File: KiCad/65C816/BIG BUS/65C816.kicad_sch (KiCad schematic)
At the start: 34 parts, among them J1 Expansion Bus, J2 Expansion Bus, J3 Expansion Bus, J4 Expansion Bus, J5 Expansion Bus, J6 Expansion Bus, J7 Displays, J8 Serial, J9 PWR IN, SW2 RESET, SW3 PWR_ON, U1 W65C816SxP, U10 74LS109, U2 HM62256BLP, U3 74HC00, U4 28C256, U5 ATF16V8B, U6 74HC245, U7 74LS573, U8 NE555P, U9 74LS109, Y1 16MHz

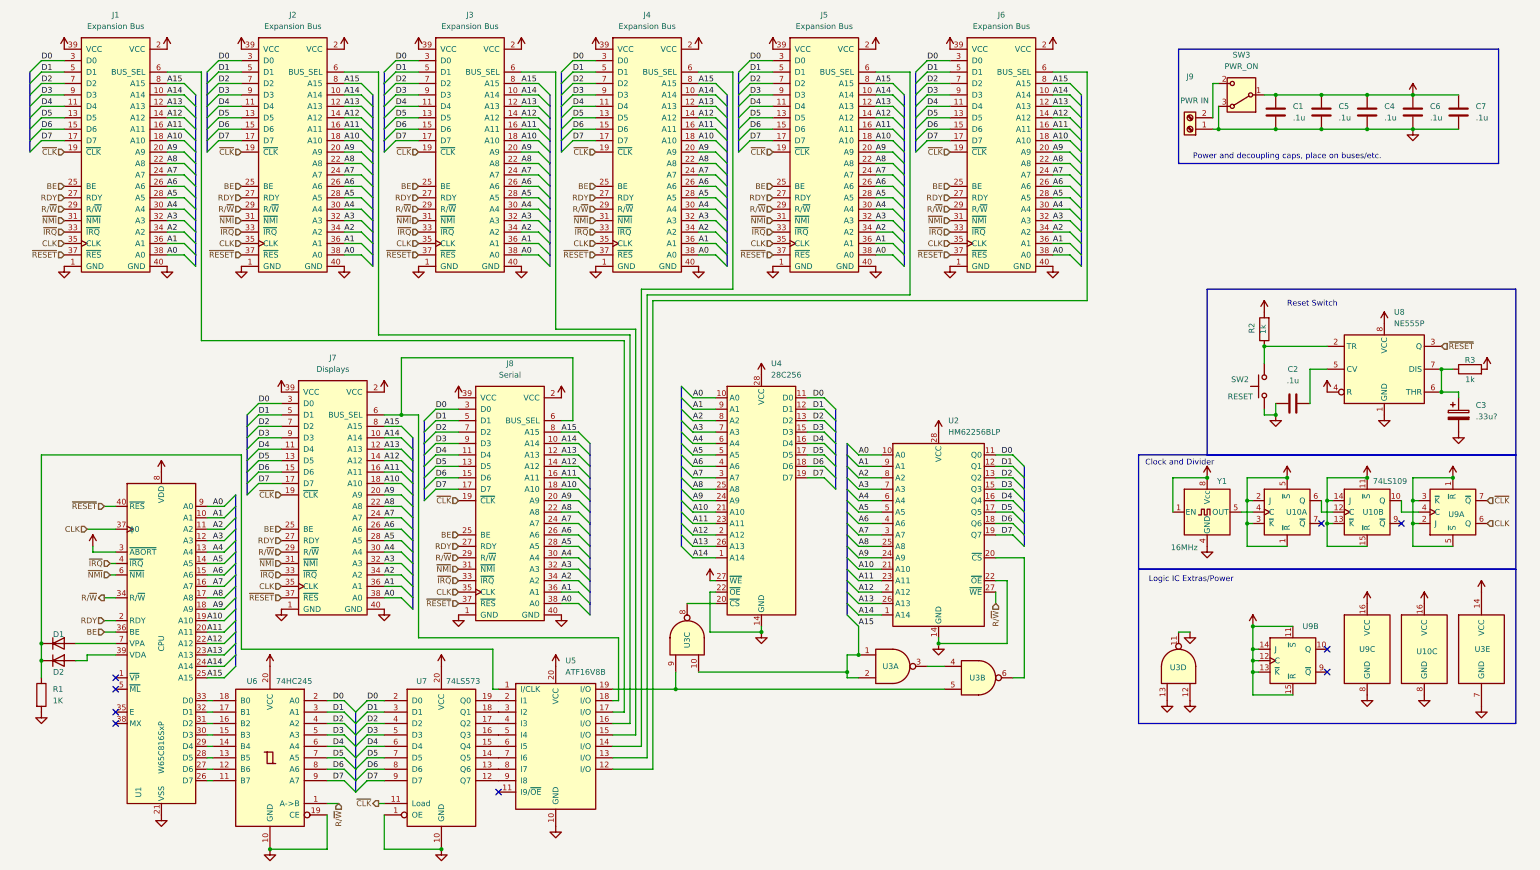
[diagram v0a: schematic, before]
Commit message: Cleaned up random files, added actual .gitignore on my end lmao
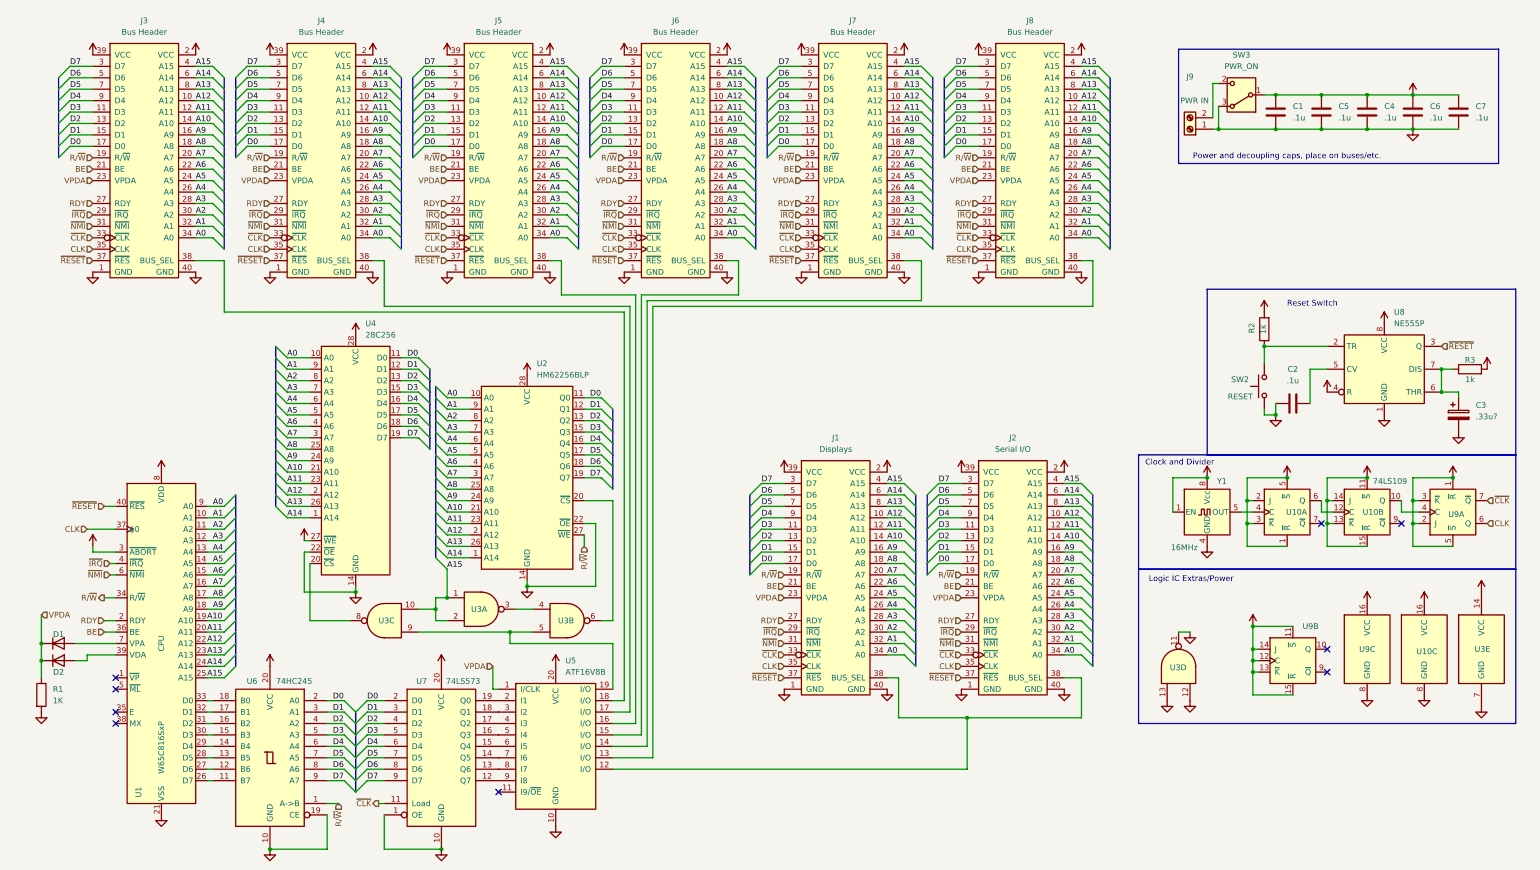
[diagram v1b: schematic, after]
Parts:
- removed J1, J2, J3, J4, J5, J6: Expansion Bus, Connector_IDC:IDC-Header_2x20_P2.54mm_Vertical, symbol Board Connectors:Generic Board Connector
- removed J7: Displays, Connector_IDC:IDC-Header_2x20_P2.54mm_Vertical, symbol Board Connectors:Generic Board Connector
- removed J8: Serial, Connector_IDC:IDC-Header_2x20_P2.54mm_Vertical, symbol Board Connectors:Generic Board Connector
- added J1: Displays, Connector_IDC:IDC-Header_2x20_P2.54mm_Vertical, symbol Board Connectors:Board_Bus_V2
- added J2: Serial I/O, Connector_IDC:IDC-Header_2x20_P2.54mm_Vertical, symbol Board Connectors:Board_Bus_V2
- added J3, J4, J5, J6, J7, J8: Bus Header, Connector_IDC:IDC-Header_2x20_P2.54mm_Vertical, symbol Board Connectors:Board_Bus_V2
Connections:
- net +5V: now also J1.2 (VCC), J1.39 (VCC), J2.2 (VCC), J2.39 (VCC), J3.2 (VCC), J3.39 (VCC), J4.2 (VCC), J4.39 (VCC), J5.2 (VCC), J5.39 (VCC), J6.2 (VCC), J6.39 (VCC), J7.2 (VCC), J7.39 (VCC), J8.2 (VCC), J8.39 (VCC)
- net A0: now also J1.34 (A0), J2.34 (A0), J3.34 (A0), J4.34 (A0), J5.34 (A0), J6.34 (A0), J7.34 (A0), J8.34 (A0)
- net A1: now also J1.32 (A1), J2.32 (A1), J3.32 (A1), J4.32 (A1), J5.32 (A1), J6.32 (A1), J7.32 (A1), J8.32 (A1)
- net A10: now also J1.14 (A10), J2.14 (A10), J3.14 (A10), J4.14 (A10), J5.14 (A10), J6.14 (A10), J7.14 (A10), J8.14 (A10)
- net A11: now also J1.12 (A11), J2.12 (A11), J3.12 (A11), J4.12 (A11), J5.12 (A11), J6.12 (A11), J7.12 (A11), J8.12 (A11)
- net A12: now also J1.10 (A12), J2.10 (A12), J3.10 (A12), J4.10 (A12), J5.10 (A12), J6.10 (A12), J7.10 (A12), J8.10 (A12)
- net A13: now also J1.8 (A13), J2.8 (A13), J3.8 (A13), J4.8 (A13), J5.8 (A13), J6.8 (A13), J7.8 (A13), J8.8 (A13)
- net A14: now also J1.6 (A14), J2.6 (A14), J3.6 (A14), J4.6 (A14), J5.6 (A14), J6.6 (A14), J7.6 (A14), J8.6 (A14)
- net A15: now also J1.4 (A15), J2.4 (A15), J3.4 (A15), J4.4 (A15), J5.4 (A15), J6.4 (A15), J7.4 (A15), J8.4 (A15)
- net A2: now also J1.30 (A2), J2.30 (A2), J3.30 (A2), J4.30 (A2), J5.30 (A2), J6.30 (A2), J7.30 (A2), J8.30 (A2)
- net A3: now also J1.28 (A3), J2.28 (A3), J3.28 (A3), J4.28 (A3), J5.28 (A3), J6.28 (A3), J7.28 (A3), J8.28 (A3)
- net A4: now also J1.26 (A4), J2.26 (A4), J3.26 (A4), J4.26 (A4), J5.26 (A4), J6.26 (A4), J7.26 (A4), J8.26 (A4)
- net A5: now also J1.24 (A5), J2.24 (A5), J3.24 (A5), J4.24 (A5), J5.24 (A5), J6.24 (A5), J7.24 (A5), J8.24 (A5)
- net A6: now also J1.22 (A6), J2.22 (A6), J3.22 (A6), J4.22 (A6), J5.22 (A6), J6.22 (A6), J7.22 (A6), J8.22 (A6)
- net A7: now also J1.20 (A7), J2.20 (A7), J3.20 (A7), J4.20 (A7), J5.20 (A7), J6.20 (A7), J7.20 (A7), J8.20 (A7)
- net A8: now also J1.18 (A8), J2.18 (A8), J3.18 (A8), J4.18 (A8), J5.18 (A8), J6.18 (A8), J7.18 (A8), J8.18 (A8)
- net A9: now also J1.16 (A9), J2.16 (A9), J3.16 (A9), J4.16 (A9), J5.16 (A9), J6.16 (A9), J7.16 (A9), J8.16 (A9)
- net BE: now also J1.21 (BE), J2.21 (BE), J3.21 (BE), J4.21 (BE), J5.21 (BE), J6.21 (BE), J7.21 (BE), J8.21 (BE)
- net CLK: now also J1.35 (CLK), J2.35 (CLK), J3.35 (CLK), J4.35 (CLK), J5.35 (CLK), J6.35 (CLK), J7.35 (CLK), J8.35 (CLK)
- net D0: now also J1.17 (D0), J2.17 (D0), J3.17 (D0), J4.17 (D0), J5.17 (D0), J6.17 (D0), J7.17 (D0), J8.17 (D0)
- net D1: now also J1.15 (D1), J2.15 (D1), J3.15 (D1), J4.15 (D1), J5.15 (D1), J6.15 (D1), J7.15 (D1), J8.15 (D1)
- net D2: now also J1.13 (D2), J2.13 (D2), J3.13 (D2), J4.13 (D2), J5.13 (D2), J6.13 (D2), J7.13 (D2), J8.13 (D2)
- net D3: now also J1.11 (D3), J2.11 (D3), J3.11 (D3), J4.11 (D3), J5.11 (D3), J6.11 (D3), J7.11 (D3), J8.11 (D3)
- net D4: now also J1.9 (D4), J2.9 (D4), J3.9 (D4), J4.9 (D4), J5.9 (D4), J6.9 (D4), J7.9 (D4), J8.9 (D4)
- net D5: now also J1.7 (D5), J2.7 (D5), J3.7 (D5), J4.7 (D5), J5.7 (D5), J6.7 (D5), J7.7 (D5), J8.7 (D5)
- net D6: now also J1.5 (D6), J2.5 (D6), J3.5 (D6), J4.5 (D6), J5.5 (D6), J6.5 (D6), J7.5 (D6), J8.5 (D6)
- net D7: now also J1.3 (D7), J2.3 (D7), J3.3 (D7), J4.3 (D7), J5.3 (D7), J6.3 (D7), J7.3 (D7), J8.3 (D7)
- net GND: now also J1.1 (GND), J1.40 (GND), J2.1 (GND), J2.40 (GND), J3.1 (GND), J3.40 (GND), J4.1 (GND), J4.40 (GND), J5.1 (GND), J5.40 (GND), J6.1 (GND), J6.40 (GND), J7.1 (GND), J7.40 (GND), J8.1 (GND), J8.40 (GND)
- net RDY: now also J1.27 (RDY), J2.27 (RDY), J3.27 (RDY), J4.27 (RDY), J5.27 (RDY), J6.27 (RDY), J7.27 (RDY), J8.27 (RDY)
- net R/~{W}: now also J1.19 (R/~{W}), J2.19 (R/~{W}), J3.19 (R/~{W}), J4.19 (R/~{W}), J5.19 (R/~{W}), J6.19 (R/~{W}), J7.19 (R/~{W}), J8.19 (R/~{W})
- net ~{CLK}: now also J1.33 (~{CLK}), J2.33 (~{CLK}), J3.33 (~{CLK}), J4.33 (~{CLK}), J5.33 (~{CLK}), J6.33 (~{CLK}), J7.33 (~{CLK}), J8.33 (~{CLK})
- net ~{IRQ}: now also J1.29 (~{IRQ}), J2.29 (~{IRQ}), J3.29 (~{IRQ}), J4.29 (~{IRQ}), J5.29 (~{IRQ}), J6.29 (~{IRQ}), J7.29 (~{IRQ}), J8.29 (~{IRQ})
- net ~{NMI}: now also J1.31 (~{NMI}), J2.31 (~{NMI}), J3.31 (~{NMI}), J4.31 (~{NMI}), J5.31 (~{NMI}), J6.31 (~{NMI}), J7.31 (~{NMI}), J8.31 (~{NMI})
- net ~{RESET}: now also J1.37 (~{RES}), J2.37 (~{RES}), J3.37 (~{RES}), J4.37 (~{RES}), J5.37 (~{RES}), J6.37 (~{RES}), J7.37 (~{RES}), J8.37 (~{RES})
- net at U5.15 (I/O): now also J6.38 (BUS_SEL)
- net at U5.18 (I/O): now also J3.38 (BUS_SEL)
- net at U5.14 (I/O): now also J7.38 (BUS_SEL)
- net at U5.12 (I/O): now also J1.38 (BUS_SEL), J2.38 (BUS_SEL)
- net at U5.16 (I/O): now also J5.38 (BUS_SEL)
- net at U5.13 (I/O): now also J8.38 (BUS_SEL)
- net VPDA: now reaches D1.1 (K), D2.1 (K), R1.1, U5.1 (I/CLK)
- net VPDA: now also J1.23 (VPDA), J2.23 (VPDA), J3.23 (VPDA), J4.23 (VPDA), J5.23 (VPDA), J6.23 (VPDA), J7.23 (VPDA), J8.23 (VPDA)
- net at U5.17 (I/O): now also J4.38 (BUS_SEL)
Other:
- moved on the sheet: U2, U3A, U3B, U3C, U4
